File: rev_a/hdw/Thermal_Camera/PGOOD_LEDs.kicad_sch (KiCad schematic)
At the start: 5 parts, among them U1501 74LVC1G97

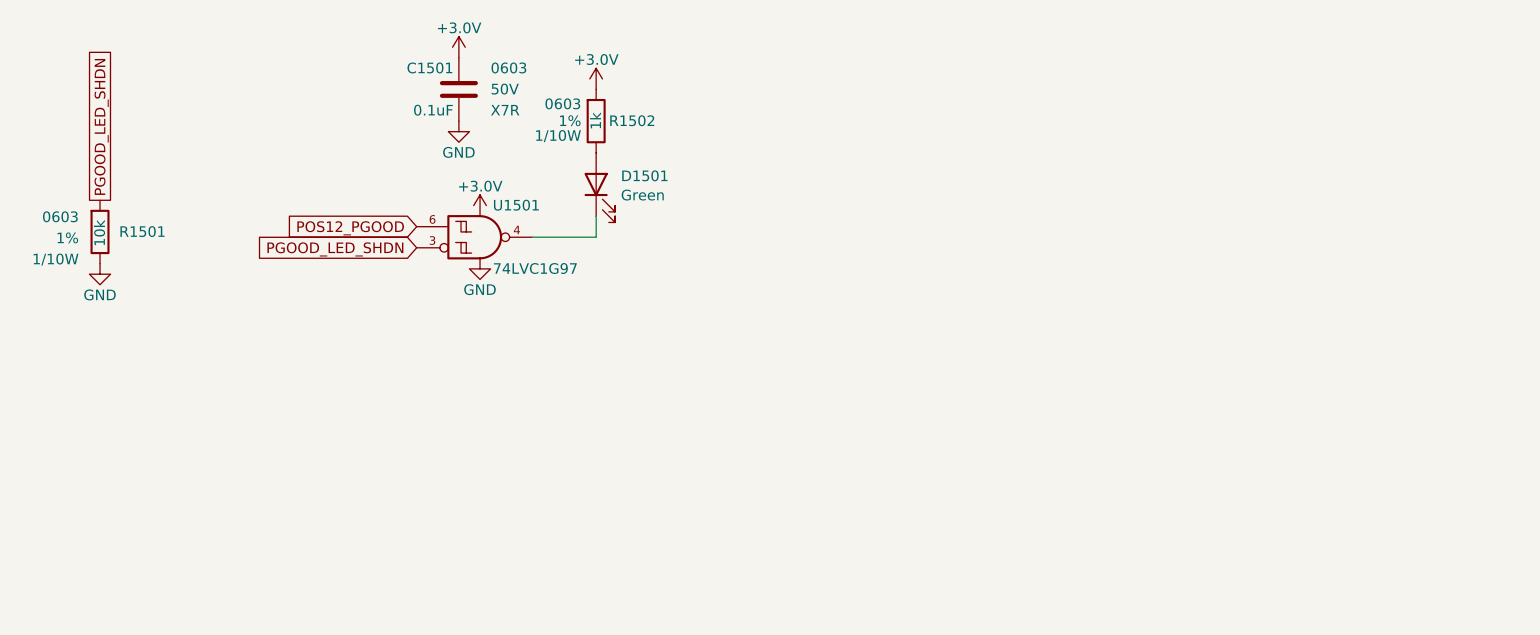
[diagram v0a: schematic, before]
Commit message: lots of random schematic progress
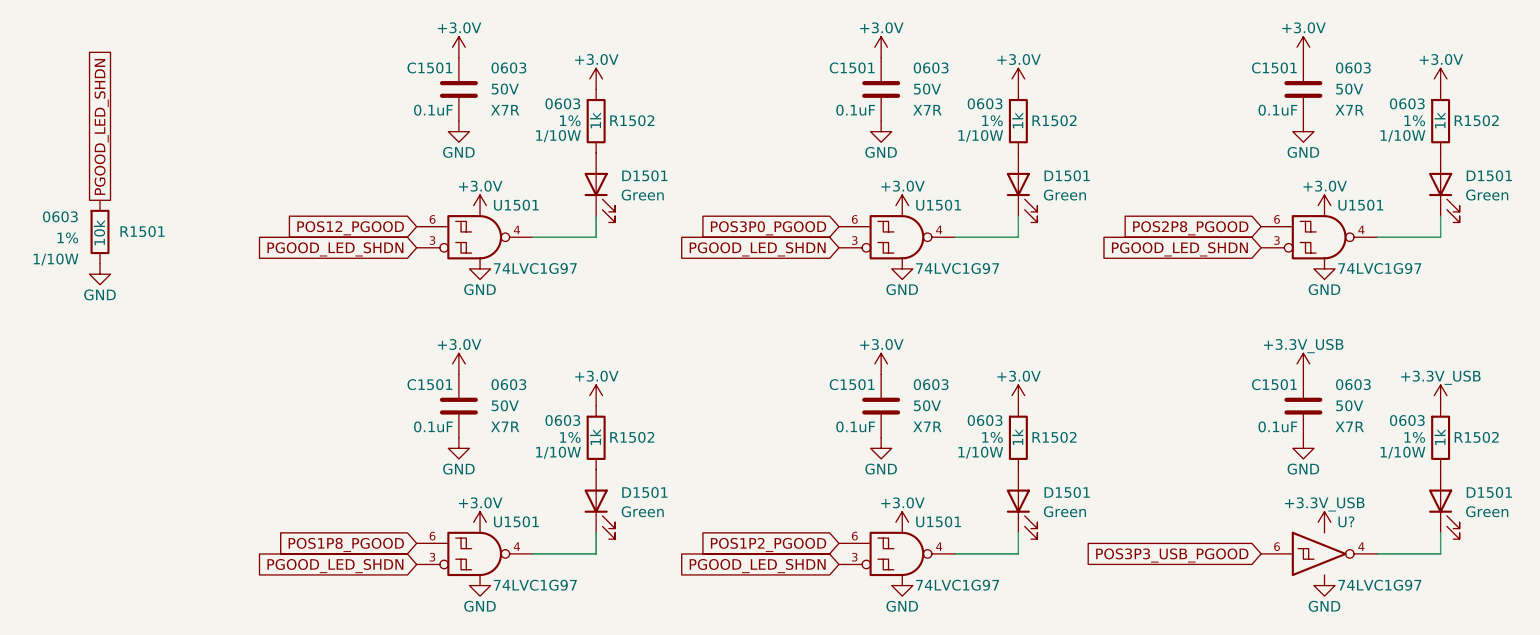
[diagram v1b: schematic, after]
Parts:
- added C1501 (x5): 0.1uF, Capacitors_SMD:C_0603, symbol Custom_Library:C_Custom
- added D1501 (x5): Green, LEDs:LED_0603, symbol Device:LED
- added R1502 (x5): 1k, Resistors_SMD:R_0603, symbol Custom_Library:R_Custom
- added U1501 (x4): 74LVC1G97, Package_TO_SOT_SMD:SOT-363_SC-70-6, symbol Custom_Library:74LVC1G97_Power_NAND_INV
- added U?: 74LVC1G97, Package_TO_SOT_SMD:SOT-363_SC-70-6, symbol Custom Library:74LVC1G97_Power_NOT
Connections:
- net +3.0V: now also C1501.1, C1501.1, C1501.1, C1501.1, R1502.1, R1502.1, R1502.1, R1502.1, U1501.1 (VCC), U1501.1 (VCC), U1501.1 (VCC), U1501.1 (VCC), U1501.5 (VCC), U1501.5 (VCC), U1501.5 (VCC), U1501.5 (VCC)
- net GND: now also C1501.2, C1501.2, C1501.2, C1501.2, C1501.2, U1501.2 (GND), U1501.2 (GND), U1501.2 (GND), U1501.2 (GND), U?.2 (GND), U?.3 (GND)
- net PGOOD_LED_SHDN: now also U1501.3, U1501.3, U1501.3, U1501.3
- new net: D1501.2 (A), R1502.2 (x5)
- new net: D1501.1 (K), U1501.4 (x4)
- new net: D1501.1 (K), U?.4
- new net +3.3V_USB: C1501.1, R1502.1, U?.1 (VCC), U?.5 (VCC)
- new net POS1P2_PGOOD: U1501.6
- new net POS1P8_PGOOD: U1501.6
- new net POS2P8_PGOOD: U1501.6
- new net POS3P0_PGOOD: U1501.6
- new net POS3P3_USB_PGOOD: U?.6
